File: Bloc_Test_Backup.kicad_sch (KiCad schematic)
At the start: 44 parts, among them Q29 2N7000, Q30 2N7000, Q31 2N7000, Q32 2N7000, Q33 2N7000, Q34 2N7000

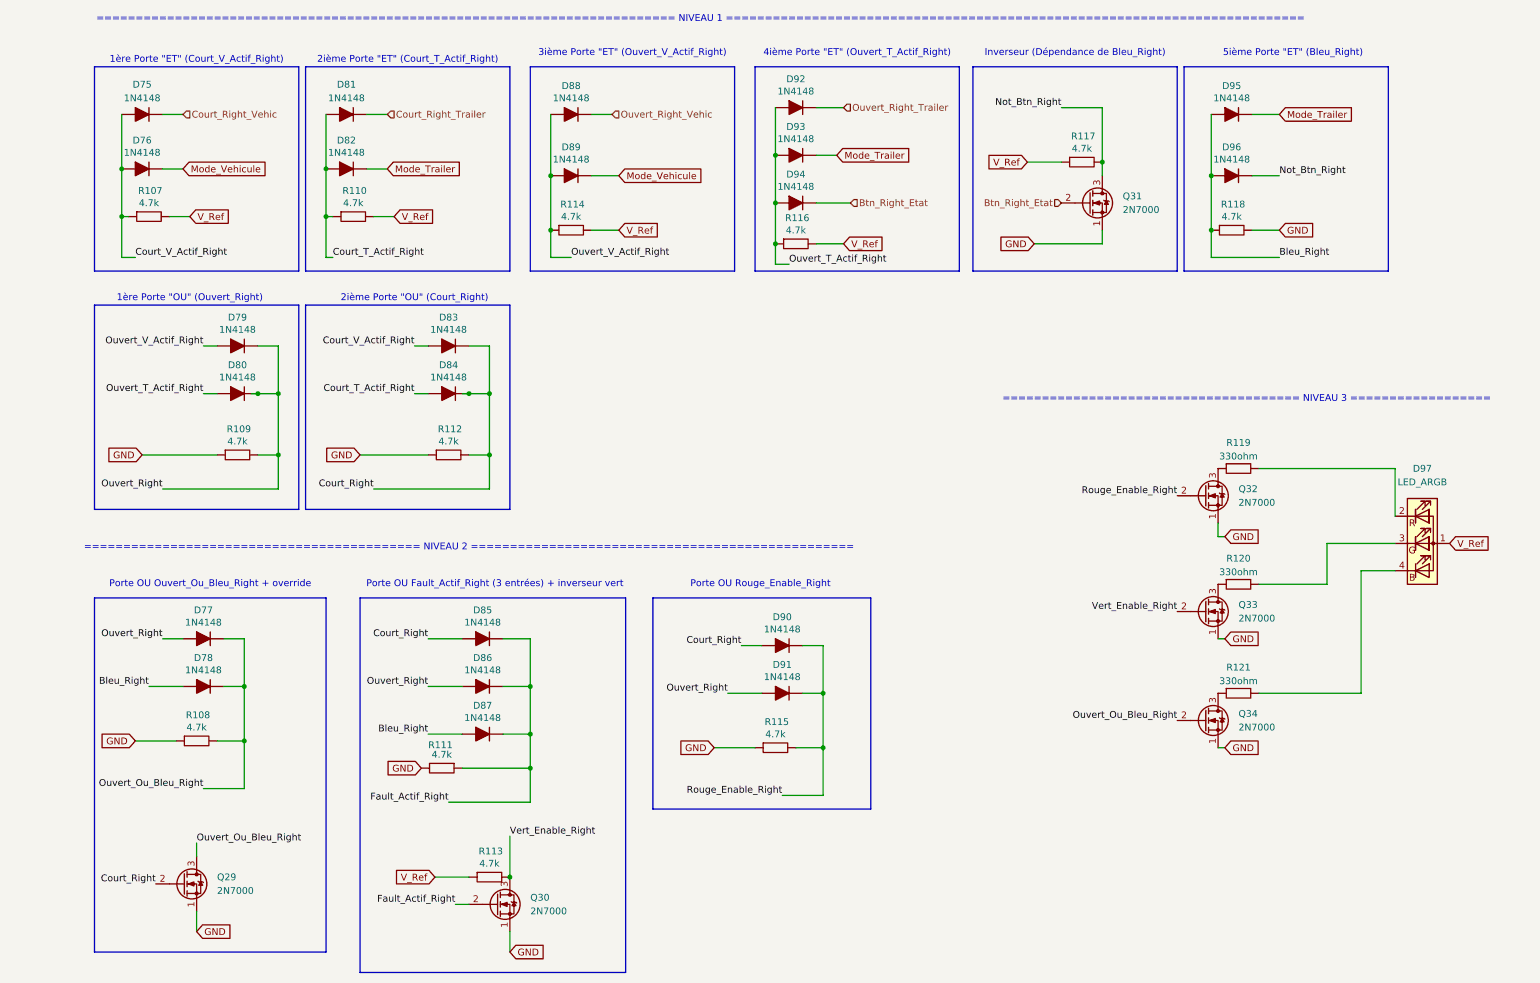
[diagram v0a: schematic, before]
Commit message: Add files via upload
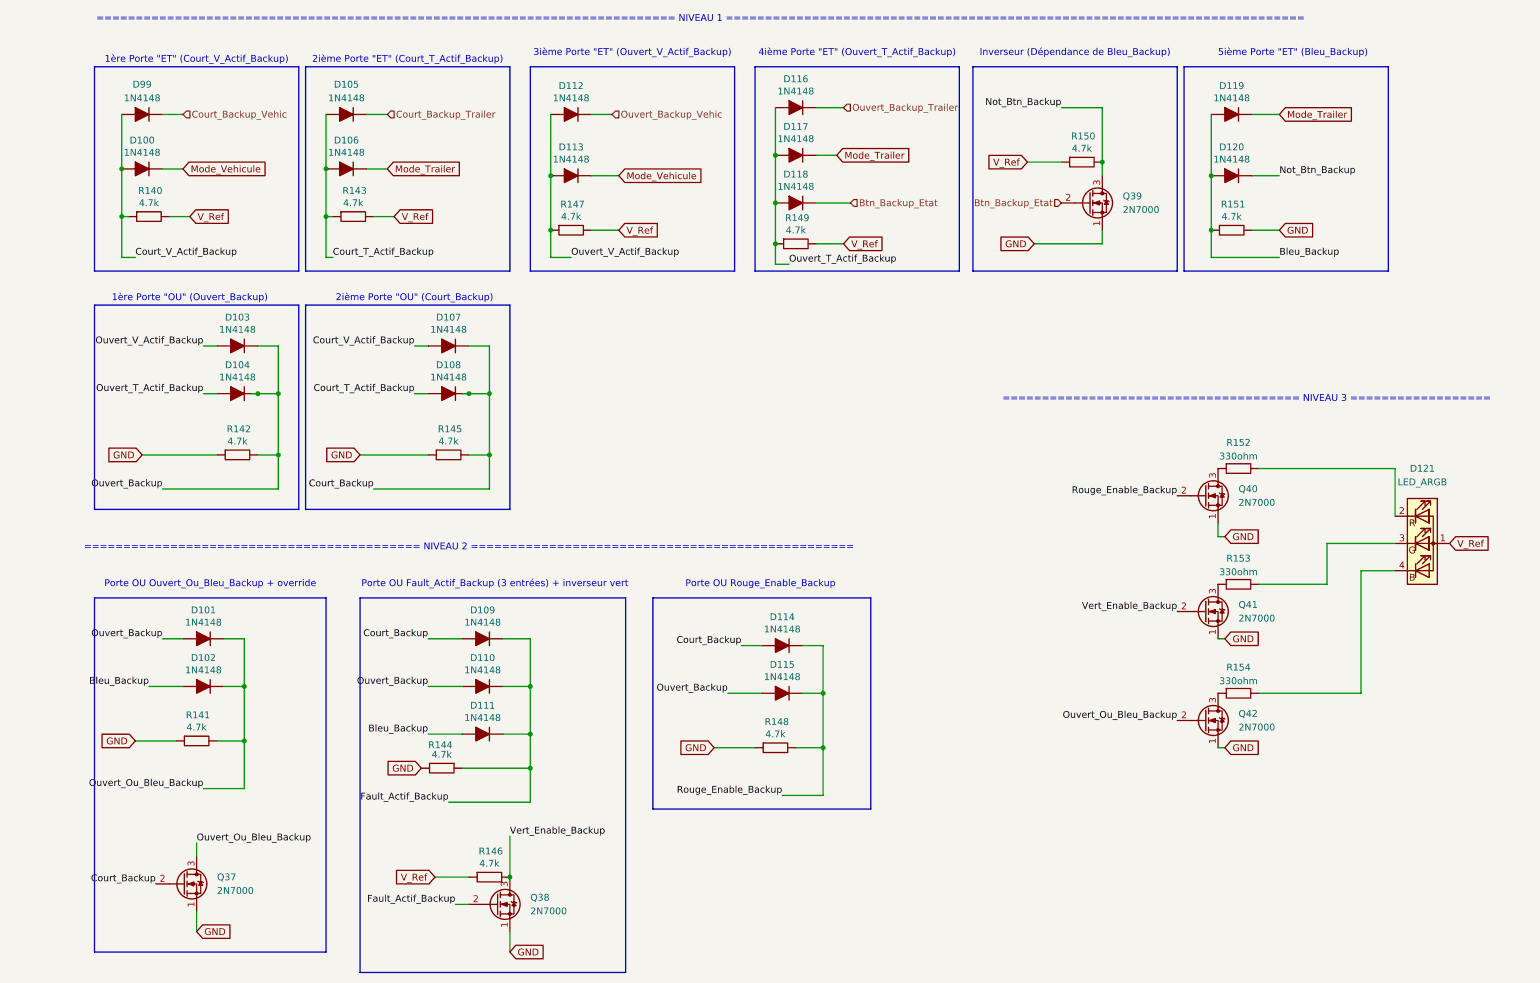
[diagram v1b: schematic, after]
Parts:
- removed D75, D76, D77, D78, D79, D80, D81, D82, D83, D84, D85, D86, D87, D88, D89, D90, D91, D92, D93, D94, D95, D96: 1N4148, PCM_Diode_THT_AKL:D_DO-35_SOD27_P7.62mm_Horizontal, symbol PCM_Diode_AKL:1N4148
- removed D97: LED_ARGB, symbol Device:LED_ARGB
- removed Q29, Q30, Q31, Q32, Q33, Q34: 2N7000, Package_TO_SOT_THT:TO-92_Inline, symbol Transistor_FET:2N7000
- removed R107, R108, R109, R110, R111, R112, R113, R114, R115, R116, R117, R118: 4.7k, Resistor_THT:R_Axial_DIN0207_L6.3mm_D2.5mm_P10.16mm_Horizontal, symbol PCM_SL_Resistors:4.7k
- removed R119, R120, R121: 330ohm, Resistor_THT:R_Axial_DIN0207_L6.3mm_D2.5mm_P10.16mm_Horizontal, symbol PCM_SL_Resistors:330ohm
- added D100, D101, D102, D103, D104, D105, D106, D107, D108, D109, D110, D111, D112, D113, D114, D115, D116, D117, D118, D119, D120, D99: 1N4148, PCM_Diode_THT_AKL:D_DO-35_SOD27_P7.62mm_Horizontal, symbol PCM_Diode_AKL:1N4148
- added D121: LED_ARGB, symbol Device:LED_ARGB
- added Q37, Q38, Q39, Q40, Q41, Q42: 2N7000, Package_TO_SOT_THT:TO-92_Inline, symbol Transistor_FET:2N7000
- added R140, R141, R142, R143, R144, R145, R146, R147, R148, R149, R150, R151: 4.7k, Resistor_THT:R_Axial_DIN0207_L6.3mm_D2.5mm_P10.16mm_Horizontal, symbol PCM_SL_Resistors:4.7k
- added R152, R153, R154: 330ohm, Resistor_THT:R_Axial_DIN0207_L6.3mm_D2.5mm_P10.16mm_Horizontal, symbol PCM_SL_Resistors:330ohm
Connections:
- net GND: now also Q37.1 (S), Q38.1 (S), Q39.1 (S), Q40.1 (S), Q41.1 (S), Q42.1 (S), R141.1, R142.1, R144.2, R145.1, R148.1, R151.2
- net Mode_Trailer: now also D106.1 (K), D117.1 (K), D119.1 (K)
- net Mode_Vehicule: now also D100.1 (K), D113.1 (K)
- net V_Ref: now also D121.1 (A), R140.2, R143.2, R146.1, R147.2, R149.2, R150.1
- new net: Q42.3 (D), R154.1
- new net: Q40.3 (D), R152.1
- new net: D121.2 (RK), R152.2
- new net: Q41.3 (D), R153.1
- new net: D121.3 (GK), R153.2
- new net: D121.4 (BK), R154.2
- new net Bleu_Backup: D102.2 (A), D111.2 (A), D119.2 (A), D120.2 (A), R151.1
- new net Btn_Backup_Etat: D118.1 (K), Q39.2 (G)
- new net Court_Backup: D107.1 (K), D108.1 (K), D109.2 (A), D114.2 (A), Q37.2 (G), R145.2
- new net Court_Backup_Trailer: D105.1 (K)
- new net Court_Backup_Vehic: D99.1 (K)
- new net Court_T_Actif_Backup: D105.2 (A), D106.2 (A), D108.2 (A), R143.1
- new net Court_V_Actif_Backup: D100.2 (A), D107.2 (A), D99.2 (A), R140.1
- new net Fault_Actif_Backup: D109.1 (K), D110.1 (K), D111.1 (K), Q38.2 (G), R144.1
- new net Not_Btn_Backup: D120.1 (K), Q39.3 (D), R150.2
- new net Ouvert_Backup: D101.2 (A), D103.1 (K), D104.1 (K), D110.2 (A), D115.2 (A), R142.2
- new net Ouvert_Backup_Trailer: D116.1 (K)
- new net Ouvert_Backup_Vehic: D112.1 (K)
- new net Ouvert_Ou_Bleu_Backup: D101.1 (K), D102.1 (K), Q37.3 (D), Q42.2 (G), R141.2
- new net Ouvert_T_Actif_Backup: D104.2 (A), D116.2 (A), D117.2 (A), D118.2 (A), R149.1
- new net Ouvert_V_Actif_Backup: D103.2 (A), D112.2 (A), D113.2 (A), R147.1
- new net Rouge_Enable_Backup: D114.1 (K), D115.1 (K), Q40.2 (G), R148.2
- new net Vert_Enable_Backup: Q38.3 (D), Q41.2 (G), R146.2
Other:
- note added: "1ère Porte "ET" (Court_V_Actif_Backup)"
- note added: "1ère Porte "OU" (Ouvert_Backup)"
- note added: "2ième Porte "ET" (Court_T_Actif_Backup)"
- note added: "2ième Porte "OU" (Court_Backup)"
- note added: "3ième Porte "ET" (Ouvert_V_Actif_Backup)"
- note added: "4ième Porte "ET" (Ouvert_T_Actif_Backup)"
- note added: "5ième Porte "ET" (Bleu_Backup)"
- note added: "Inverseur (Dépendance de Bleu_Backup)"
- note added: "Porte OU Fault_Actif_Backup (3 entrées) + inverseur vert"
- note added: "Porte OU Ouvert_Ou_Bleu_Backup + override"
- note added: "Porte OU Rouge_Enable_Backup"
- note removed: "1ère Porte "ET" (Court_V_Actif_Right)"
- note removed: "1ère Porte "OU" (Ouvert_Right)"
- note removed: "2ième Porte "ET" (Court_T_Actif_Right)"
- note removed: "2ième Porte "OU" (Court_Right)"
- note removed: "3ième Porte "ET" (Ouvert_V_Actif_Right)"
- note removed: "4ième Porte "ET" (Ouvert_T_Actif_Right)"
- note removed: "5ième Porte "ET" (Bleu_Right)"
- note removed: "Inverseur (Dépendance de Bleu_Right)"
- note removed: "Porte OU Fault_Actif_Right (3 entrées) + inverseur vert"
- note removed: "Porte OU Ouvert_Ou_Bleu_Right + override"
- note removed: "Porte OU Rouge_Enable_Right"

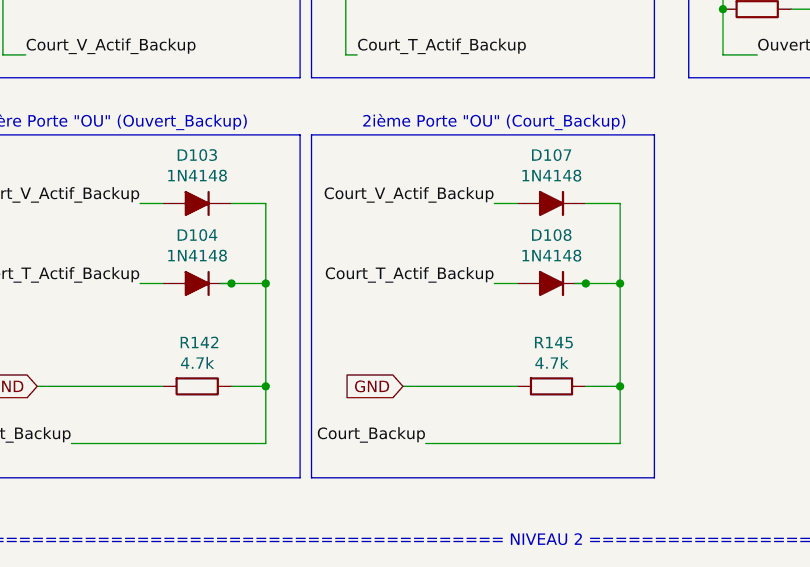
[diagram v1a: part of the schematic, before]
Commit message: Add files via upload
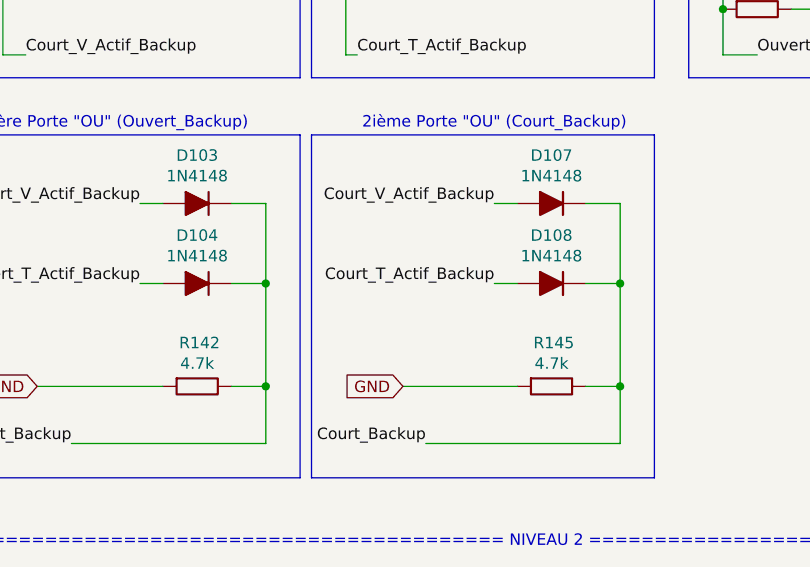
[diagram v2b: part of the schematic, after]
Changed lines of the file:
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@@
 	)
 	(junction
-		(at 52.07 86.36)
+		(at 229.87 55.88)
+		(diameter 0)
+		(color 0 0 0 0)
+	)
+	(junction
+		(at 102.87 156.21)
+		(diameter 0)
+		(color 0 0 0 0)
+	)
+	(junction
+		(at 106.68 45.72)
+		(diameter 0)
+		(color 0 0 0 0)
+	)
+	(junction
+		(at 26.67 44.45)
+		(diameter 0)
+		(color 0 0 0 0)
+	)
+	(junction
+		(at 148.59 58.42)
+		(diameter 0)
+		(color 0 0 0 0)
+	)
+	(junction
+		(at 148.59 41.91)
+		(diameter 0)
+		(color 0 0 0 0)
+	)
+	(junction
+		(at 148.59 50.8)
+		(diameter 0)
+		(color 0 0 0 0)
+	)
+	(junction
+		(at 106.68 55.88)
+		(diameter 0)
+		(color 0 0 0 0)
+	)
+	(junction
+		(at 99.06 176.53)
+		(diameter 0)
+		(color 0 0 0 0)
+	)
+	(junction
+		(at 64.77 44.45)
+		(diameter 0)
+		(color 0 0 0 0)
+	)
+	(junction
+		(at 102.87 140.97)
+		(diameter 0)
+		(color 0 0 0 0)
+	)
+	(junction
+		(at 157.48 152.4)
 		(diameter 0)
 		(color 0 0 0 0)
@@
 	)
 	(junction
-		(at 229.87 55.88)
-		(diameter 0)
-		(color 0 0 0 0)
-	)
-	(junction
-		(at 102.87 156.21)
-		(diameter 0)
-		(color 0 0 0 0)
-	)
-	(junction
-		(at 106.68 45.72)
-		(diameter 0)
-		(color 0 0 0 0)
-	)
-	(junction
-		(at 26.67 44.45)
-		(diameter 0)
-		(color 0 0 0 0)
-	)
-	(junction
-		(at 148.59 58.42)
-		(diameter 0)
-		(color 0 0 0 0)
-	)
-	(junction
-		(at 148.59 41.91)
-		(diameter 0)
-		(color 0 0 0 0)
-	)
-	(junction
-		(at 148.59 50.8)
-		(diameter 0)
-		(color 0 0 0 0)
-	)
-	(junction
-		(at 106.68 55.88)
-		(diameter 0)
-		(color 0 0 0 0)
-	)
-	(junction
-		(at 99.06 176.53)
-		(diameter 0)
-		(color 0 0 0 0)
-	)
-	(junction
-		(at 64.77 44.45)
-		(diameter 0)
-		(color 0 0 0 0)
-	)
-	(junction
-		(at 102.87 140.97)
-		(diameter 0)
-		(color 0 0 0 0)
-	)
-	(junction
-		(at 157.48 152.4)
-		(diameter 0)
-		(color 0 0 0 0)
-	)
-	(junction
 		(at 49.53 151.13)
 		(diameter 0)
@@
 	)
 	(junction
-		(at 91.44 86.36)
-		(diameter 0)
-		(color 0 0 0 0)
-	)
-	(junction
 		(at 157.48 142.24)
 		(diameter 0)
@@
 	(wire
 		(pts
-			(xy 50.8 86.36) (xy 52.07 86.36)
-		)
-		(stroke
-			(width 0)
-			(type default)
-		)
-	)
-	(wire
-		(pts
 			(xy 156.21 33.02) (xy 161.29 33.02)
 		)
@@
 	(wire
 		(pts
+			(xy 55.88 86.36) (xy 55.88 97.79)
+		)
+		(stroke
+			(width 0)
+			(type default)
+		)
+	)
+	(wire
+		(pts
 			(xy 137.16 152.4) (xy 144.78 152.4)
 		)
@@
 	(wire
 		(pts
-			(xy 90.17 86.36) (xy 91.44 86.36)
-		)
-		(stroke
-			(width 0)
-			(type default)
-		)
-	)
-	(wire
-		(pts
 			(xy 95.25 77.47) (xy 91.44 77.47)
 		)
@@
 	(wire
 		(pts
-			(xy 55.88 86.36) (xy 52.07 86.36)
-		)
-		(stroke
-			(width 0)
-			(type default)
-		)
-	)
-	(wire
-		(pts
 			(xy 26.67 53.34) (xy 27.94 53.34)
 		)
@@
 	(wire
 		(pts
-			(xy 55.88 86.36) (xy 55.88 97.79)
-		)
-		(stroke
+			(xy 52.07 86.36) (xy 55.88 86.36)
+		)
+		(stroke
